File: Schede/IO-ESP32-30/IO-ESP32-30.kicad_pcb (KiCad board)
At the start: 2 copper layers, 60 parts, among them Q1 IRF540N, Q2 IRF540N, Q3 IRF540N, Q4 IRF540N, Q5 IRF540N, Q6 IRF540N, Q7 IRF540N, Q8 IRF540N, U1 L7805, U2 DOIT-ESP32-30PIN

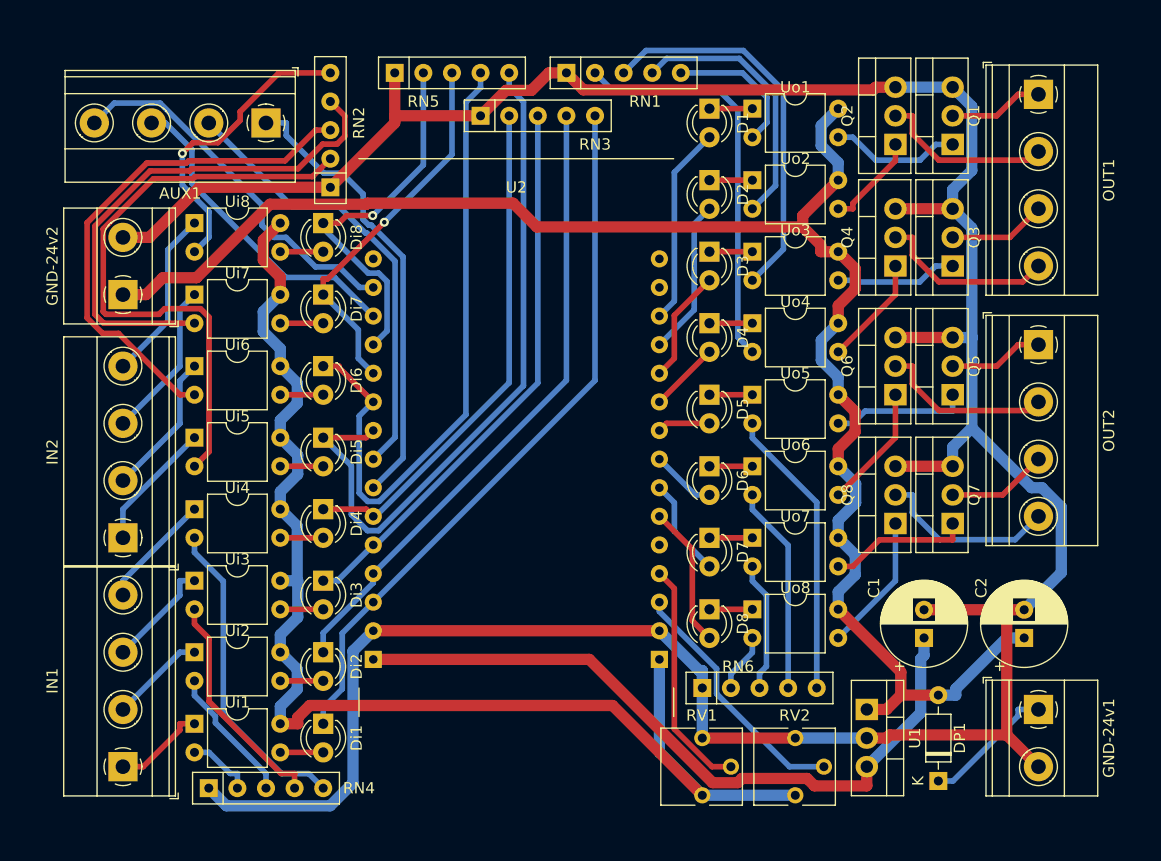
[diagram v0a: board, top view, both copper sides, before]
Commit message: ok
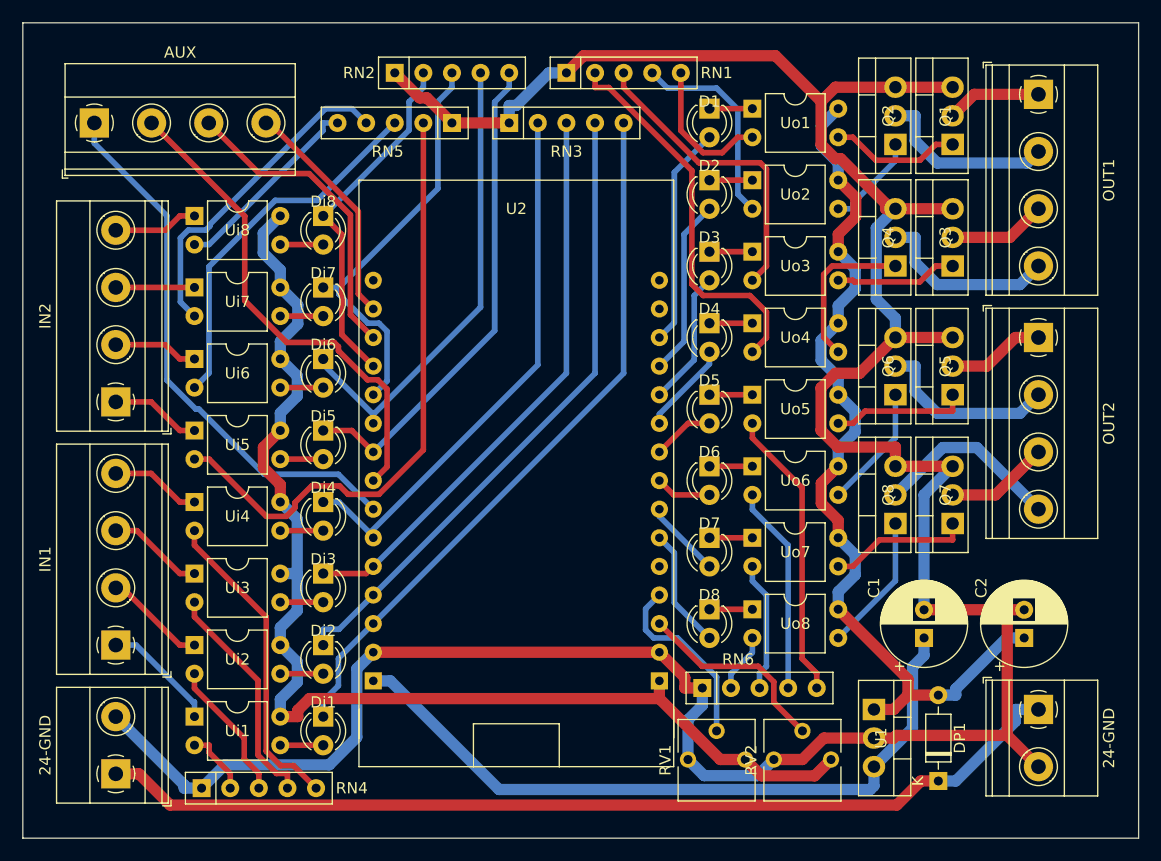
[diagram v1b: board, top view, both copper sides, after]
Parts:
- removed GND-24v1: Screw_Terminal_01x02, TerminalBlock_Phoenix:TerminalBlock_Phoenix_MKDS-1,5-2-5.08_1x02_P5.08mm_Horizontal
- added 24-GND: Screw_Terminal_01x02, TerminalBlock_Phoenix:TerminalBlock_Phoenix_MKDS-1,5-2-5.08_1x02_P5.08mm_Horizontal, F.Cu at (90.2, 61.0)
- moved 24-GND 42.5 mm to (8.26, 66.7)
- moved AUX 15.2 mm to (6.35, 8.89), turned to 0 degrees
- moved RN2 12.2 mm to (38.1, 8.89), turned to 180 degrees
- moved IN2 12.1 mm to (8.26, 33.7)
- moved IN1 10.8 mm to (8.26, 55.2)
- moved RV1 4.96 mm to (64.1, 65.4), turned to 90 degrees
- moved RV2 4.49 mm to (71.8, 65.4), turned to 90 degrees
- moved RN3 2.62 mm to (43.2, 8.89)
- moved U2 1.91 mm to (43.8, 16.5)
- moved Di2 0.64 mm to (26.7, 55.2)
- moved Ui2 0.64 mm to (15.2, 55.2)
- moved Di6 0.64 mm to (26.7, 29.8)
- moved Di8 0.64 mm to (26.7, 17.1)
- moved RN4 0.64 mm to (15.9, 67.9)
- moved Ui6 0.64 mm to (15.2, 29.8)
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- renumbered GND-24v2 to 24-GND, AUX1 to AUX
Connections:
- net Net-(OUT1-Pad1) renamed /P1
- net Net-(OUT1-Pad2) renamed /P2
- net Net-(OUT1-Pad3) renamed /P3
- net Net-(OUT1-Pad4) renamed /P4
- net Net-(OUT2-Pad1) renamed /P5
- net Net-(OUT2-Pad2) renamed /P6
- net Net-(OUT2-Pad3) renamed /P7
- net Net-(OUT2-Pad4) renamed /P8
- 24-GND pad 1: +24V -> VCC
- DP1 pad 1: Net-(DP1-Pad1) -> VCC
- U2 pad 1: Net-(U2-Pad1) -> (no net)
- U2 pad 20: Net-(U2-Pad20) -> (no net)
- U2 pad 29: Net-(U2-Pad29) -> (no net)
- U2 pad 30: Net-(U2-Pad30) -> (no net)
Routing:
- net VCC: track 0.00 -> 87.2 mm
- net +24V: track 146.9 -> 79.7 mm
- net Net-(Di5-Pad1): track 62.1 -> 43.9 mm
- net Net-(RN2-Pad4): track 46.1 -> 29.3 mm
- net Net-(Di6-Pad1): track 58.3 -> 41.8 mm
- net GND: track 275.8 -> 259.6 mm
- net Net-(RN2-Pad3): track 45.8 -> 33.0 mm
- net Net-(AUX1-Pad4): track 33.3 -> 20.6 mm
- net Net-(DP1-Pad1): track 11.8 -> 0.00 mm
- net Net-(RN2-Pad5): track 26.8 -> 17.6 mm, vias 1 -> 0
- net +3V3: track 117.2 -> 108.4 mm
- net Net-(AUX1-Pad1): track 40.7 -> 48.6 mm
- net Net-(IN2-Pad4): track 15.3 -> 7.51 mm
- net Net-(RN1-Pad3): track 34.5 -> 27.4 mm
- net Net-(IN2-Pad3): track 14.1 -> 6.98 mm
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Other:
- board outline added: 99.1 x 72.4 mm
